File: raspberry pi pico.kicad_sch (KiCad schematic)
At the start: 11 parts, among them J1 USB_OTG, U1 RP2350A, U2 RT6150B-33GQW

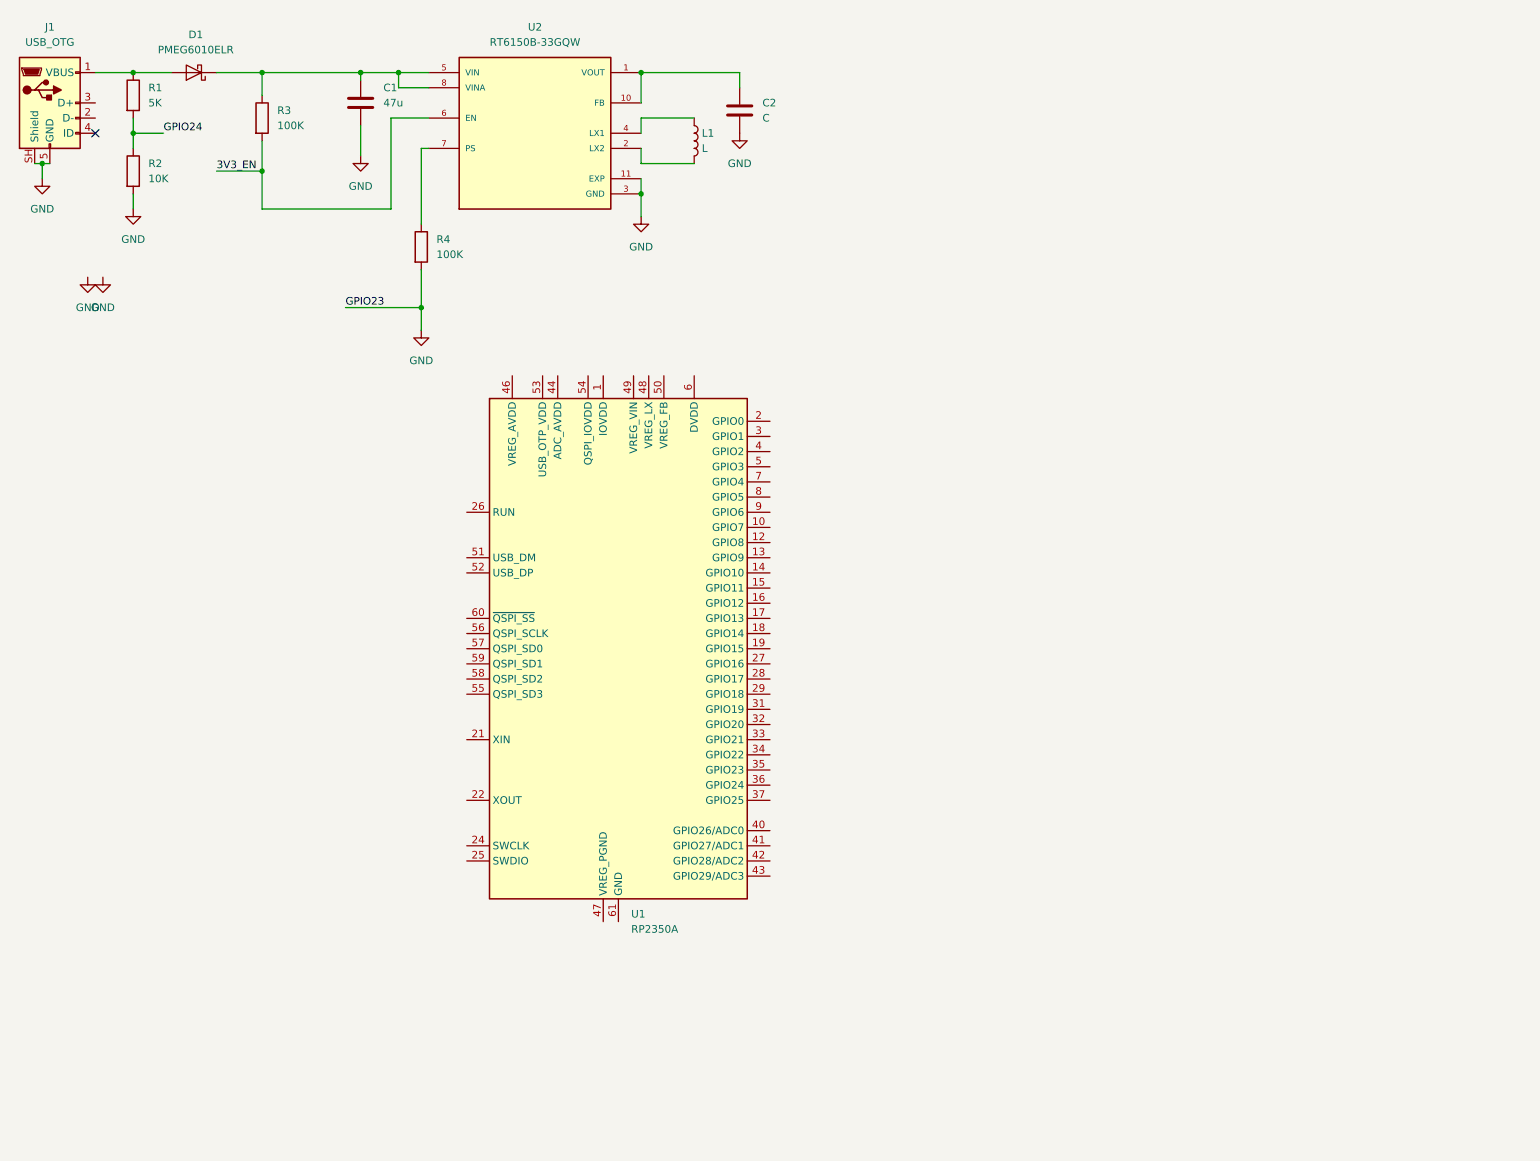
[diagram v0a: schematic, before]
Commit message: Add files via upload
these files present my progress comparing to the 1st upload
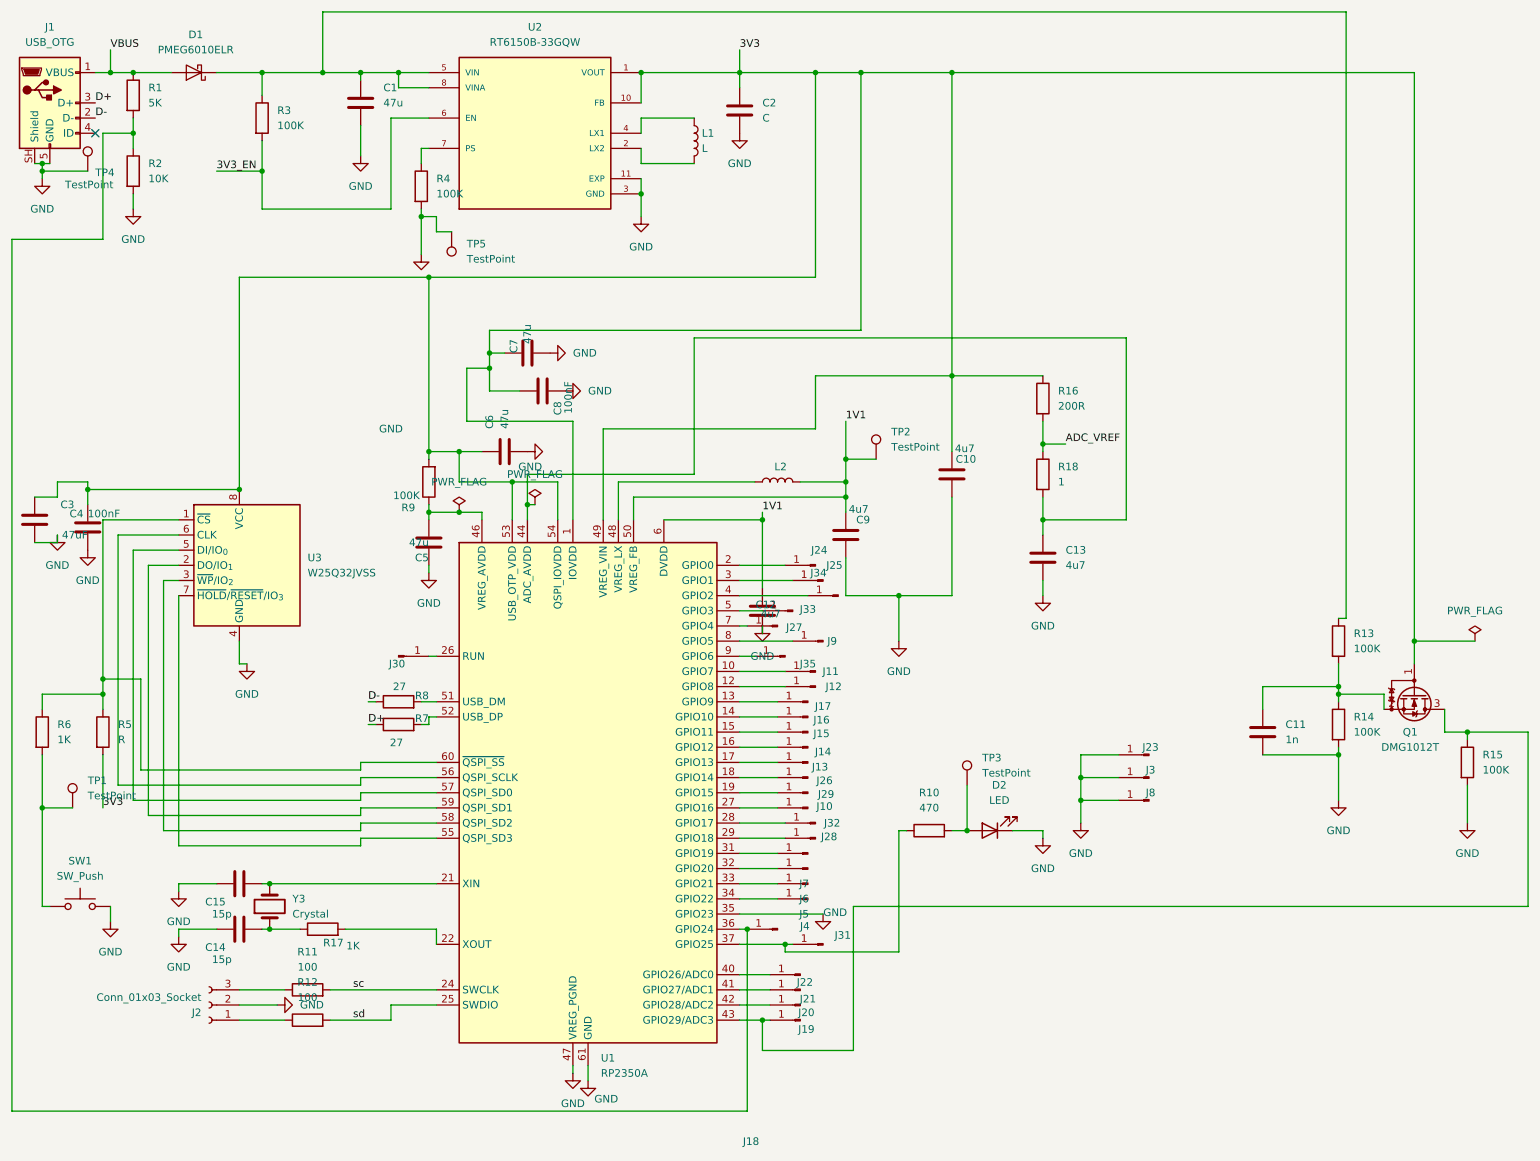
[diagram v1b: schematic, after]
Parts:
- added C10, C12, C13, C9: 4u7, Capacitor_SMD:C_0805_2012Metric_Pad1.18x1.45mm_HandSolder, symbol Device:C
- added C11: 1n, Capacitor_SMD:C_0805_2012Metric_Pad1.18x1.45mm_HandSolder, symbol Device:C
- added C14, C15: 15p, Capacitor_SMD:C_0805_2012Metric_Pad1.18x1.45mm_HandSolder, symbol Device:C
- added C3: 47uF, Capacitor_SMD:C_0805_2012Metric_Pad1.18x1.45mm_HandSolder, symbol Device:C
- added C4, C8: 100nF, Capacitor_SMD:C_0805_2012Metric_Pad1.18x1.45mm_HandSolder, symbol Device:C
- added C5, C6, C7: 47u, Capacitor_SMD:C_0805_2012Metric_Pad1.18x1.45mm_HandSolder, symbol Device:C
- added D2: LED, LED_THT:LED_D3.0mm, symbol Device:LED
- added J10, J11, J12, J13, J14, J15, J16, J17, J18, J19, J20, J21, J22, J23, J24, J25, J26, J27, J28, J29, J3, J30, J31, J32, J33, J34, J35, J4, J5, J6, J7, J8, J9: Conn_01x01_Pin, Connector_PinHeader_1.00mm:PinHeader_1x01_P1.00mm_Vertical, symbol Connector:Conn_01x01_Pin
- added J2: Conn_01x03_Socket, Connector_PinHeader_1.00mm:PinHeader_1x03_P1.00mm_Horizontal, symbol Connector:Conn_01x03_Socket
- added L2: 3u3, Inductor_SMD:L_01005_0402Metric, symbol Device:L
- added Q1: DMG1012T, Package_TO_SOT_SMD:SOT-523, symbol Transistor_FET:DMG1012T
- added R10: 470, Resistor_SMD:R_0603_1608Metric_Pad0.98x0.95mm_HandSolder, symbol Device:R
- added R11, R12: 100, Resistor_SMD:R_0603_1608Metric_Pad0.98x0.95mm_HandSolder, symbol Device:R
- added R13, R14, R15, R9: 100K, Resistor_SMD:R_0603_1608Metric_Pad0.98x0.95mm_HandSolder, symbol Device:R
- added R16: 200R, Resistor_SMD:R_0603_1608Metric_Pad0.98x0.95mm_HandSolder, symbol Device:R
- added R17, R6: 1K, Resistor_SMD:R_0603_1608Metric_Pad0.98x0.95mm_HandSolder, symbol Device:R
- added R18: 1, Resistor_SMD:R_0603_1608Metric_Pad0.98x0.95mm_HandSolder, symbol Device:R
- added R5: R, Resistor_SMD:R_0603_1608Metric_Pad0.98x0.95mm_HandSolder, symbol Device:R
- added R7, R8: 27, Resistor_SMD:R_0603_1608Metric_Pad0.98x0.95mm_HandSolder, symbol Device:R
- added SW1: SW_Push, Button_Switch_THT:SW_PUSH_6mm, symbol Switch:SW_Push
- added TP1, TP2, TP3, TP4, TP5: TestPoint, TestPoint:TestPoint_Bridge_Pitch2.54mm_Drill1.0mm, symbol Connector:TestPoint
- added U3: W25Q32JVSS, Package_SO:SOIC-8_5.3x5.3mm_P1.27mm, symbol Memory_Flash:W25Q32JVSS
- added Y3: Crystal, Crystal:Crystal_AT310_D3.0mm_L10.0mm_Horizontal, symbol Device:Crystal
- C1, C2: footprint (none) -> Capacitor_SMD:C_0805_2012Metric_Pad1.18x1.45mm_HandSolder
- J1: footprint Connector_USB:USB_Micro-B_Amphenol_10103594-0001LF_Horizontal -> Connector_USB:USB_Micro-B_Amphenol_10118194_Horizontal
- L1: footprint (none) -> Inductor_SMD:L_01005_0402Metric
- R1, R2, R3, R4: footprint (none) -> Resistor_SMD:R_0603_1608Metric_Pad0.98x0.95mm_HandSolder
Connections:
- net GPIO24 is gone; now on an unnamed net: R1.2, R2.1
- net GND: now also U1.35 (GPIO23), U1.47 (VREG_PGND), U1.61 (GND), C10.1, C11.2, C12.1, C13.2, C14.1, C15.1, C3.2, C4.2, C5.1, C6.2, C7.2, C8.2, C9.1, D2.1 (K), J2.2 (Pin_2), J23.1 (Pin_1), J3.1 (Pin_1), J8.1 (Pin_1), R14.2, R15.2, SW1.2, TP4.1, TP5.1, U3.4 (GND)
- net 3V3: now reaches C2.1, U2.1 (VOUT), U2.10 (FB)
- net 3V3: now also U1.1 (IOVDD), U1.11 (IOVDD), U1.20 (IOVDD), U1.30 (IOVDD), U1.38 (IOVDD), U1.45 (IOVDD), U1.49 (VREG_VIN), U1.53 (USB_OTP_VDD), U1.54 (QSPI_IOVDD), C10.2, C3.1, C4.1, C6.1, C7.1, C8.1, Q1.1 (G), R16.1, R5.2, R9.2, U3.8 (VCC)
- net at C1.1, D1.1 (K), R3.1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: now also R13.1
- net VBUS: now reaches D1.2 (A), J1.1 (VBUS), R1.1
- net at U1.10 (GPIO7): now also J11.1 (Pin_1)
- net at U1.12 (GPIO8): now also J12.1 (Pin_1)
- net at U1.13 (GPIO9): now also J17.1 (Pin_1)
- net at U1.14 (GPIO10): now also J16.1 (Pin_1)
- net at U1.15 (GPIO11): now also J15.1 (Pin_1)
- net at U1.16 (GPIO12): now also J14.1 (Pin_1)
- net at U1.17 (GPIO13): now also J13.1 (Pin_1)
- net at U1.18 (GPIO14): now also J26.1 (Pin_1)
- net at U1.19 (GPIO15): now also J29.1 (Pin_1)
- net at U1.2 (GPIO0): now also J34.1 (Pin_1)
- net at U1.21 (XIN): now also C15.2, Y3.2
- net at U1.22 (XOUT): now also R17.2
- net 1V1: now reaches U1.23 (DVDD), U1.39 (DVDD), U1.6 (DVDD)
- net 1V1: now also U1.50 (VREG_FB), C12.2, C9.2, L2.2, TP2.1
- net sc: now reaches U1.24 (SWCLK)
- net sc: now also R11.2
- net sd: now reaches U1.25 (SWDIO)
- net sd: now also R12.2
- net at U1.26 (RUN): now also J30.1 (Pin_1)
- net at U1.27 (GPIO16): now also J10.1 (Pin_1)
- net at U1.28 (GPIO17): now also J32.1 (Pin_1)
- net at U1.29 (GPIO18): now also J28.1 (Pin_1)
- net at U1.3 (GPIO1): now also J24.1 (Pin_1)
- net at U1.31 (GPIO19): now also J7.1 (Pin_1)
- net at U1.32 (GPIO20): now also J6.1 (Pin_1)
- net at U1.33 (GPIO21): now also J5.1 (Pin_1)
- net at U1.34 (GPIO22): now also J4.1 (Pin_1)
- net at U1.36 (GPIO24): now also J18.1 (Pin_1)
- net at U1.37 (GPIO25): now also J31.1 (Pin_1), R10.1
- net at U1.4 (GPIO2): now also J25.1 (Pin_1)
- net at U1.40 (GPIO26/ADC0): now also J22.1 (Pin_1)
- net at U1.41 (GPIO27/ADC1): now also J21.1 (Pin_1)
- net at U1.42 (GPIO28/ADC2): now also J20.1 (Pin_1)
- net at U1.43 (GPIO29/ADC3): now also J19.1 (Pin_1), Q1.3 (D), R15.1
- net at U1.44 (ADC_AVDD): now also C13.1, R18.2
- net at U1.46 (VREG_AVDD): now also C5.2, R9.1
- net at U1.48 (VREG_LX): now also L2.1
- net at U1.5 (GPIO3): now also J33.1 (Pin_1)
- net at U1.51 (USB_DM): now also R8.2
- net at U1.52 (USB_DP): now also R7.2
- net at U1.55 (QSPI_SD3): now also U3.7 (~{HOLD}/~{RESET}/IO_{3})
- net at U1.56 (QSPI_SCLK): now also U3.6 (CLK)
- net at U1.57 (QSPI_SD0): now also U3.5 (DI/IO_{0})
- net at U1.58 (QSPI_SD2): now also U3.3 (~{WP}/IO_{2})
- net at U1.59 (QSPI_SD1): now also U3.2 (DO/IO_{1})
- net at U1.60 (~{QSPI_SS}): now also R5.1, R6.1, U3.1 (~{CS})
- net at U1.7 (GPIO4): now also J27.1 (Pin_1)
- net at U1.8 (GPIO5): now also J9.1 (Pin_1)
- net at U1.9 (GPIO6): now also J35.1 (Pin_1)
- net D-: now reaches J1.2 (D-)
- net D-: now also R8.1
- net D+: now reaches J1.3 (D+)
- net D+: now also R7.1
- new net: R6.2, SW1.1, TP1.1
- new net: J2.1 (Pin_1), R12.1
- new net: D2.2 (A), R10.2, TP3.1
- new net: C11.1, Q1.2 (S), R13.2, R14.1
- new net: C14.2, R17.1, Y3.1
- new net: J2.3 (Pin_3), R11.1
- new net ADC_VREF: R16.2, R18.1
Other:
- moved on the sheet: R4, U1
